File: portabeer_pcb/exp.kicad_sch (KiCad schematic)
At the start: 34 parts, among them J16 Conn_01x03, J18 Conn_02x05_Odd_Even, J4 Conn_01x08, M1 Air pump, Q6 SiS454DN, U12 PCA9536DP, U13 USBLC6-2SC6, U16 MCP47FEB12, U17 REF3012, U18 USBLC6-4SC6, U19 FDC1004DGST, U4 COS1416

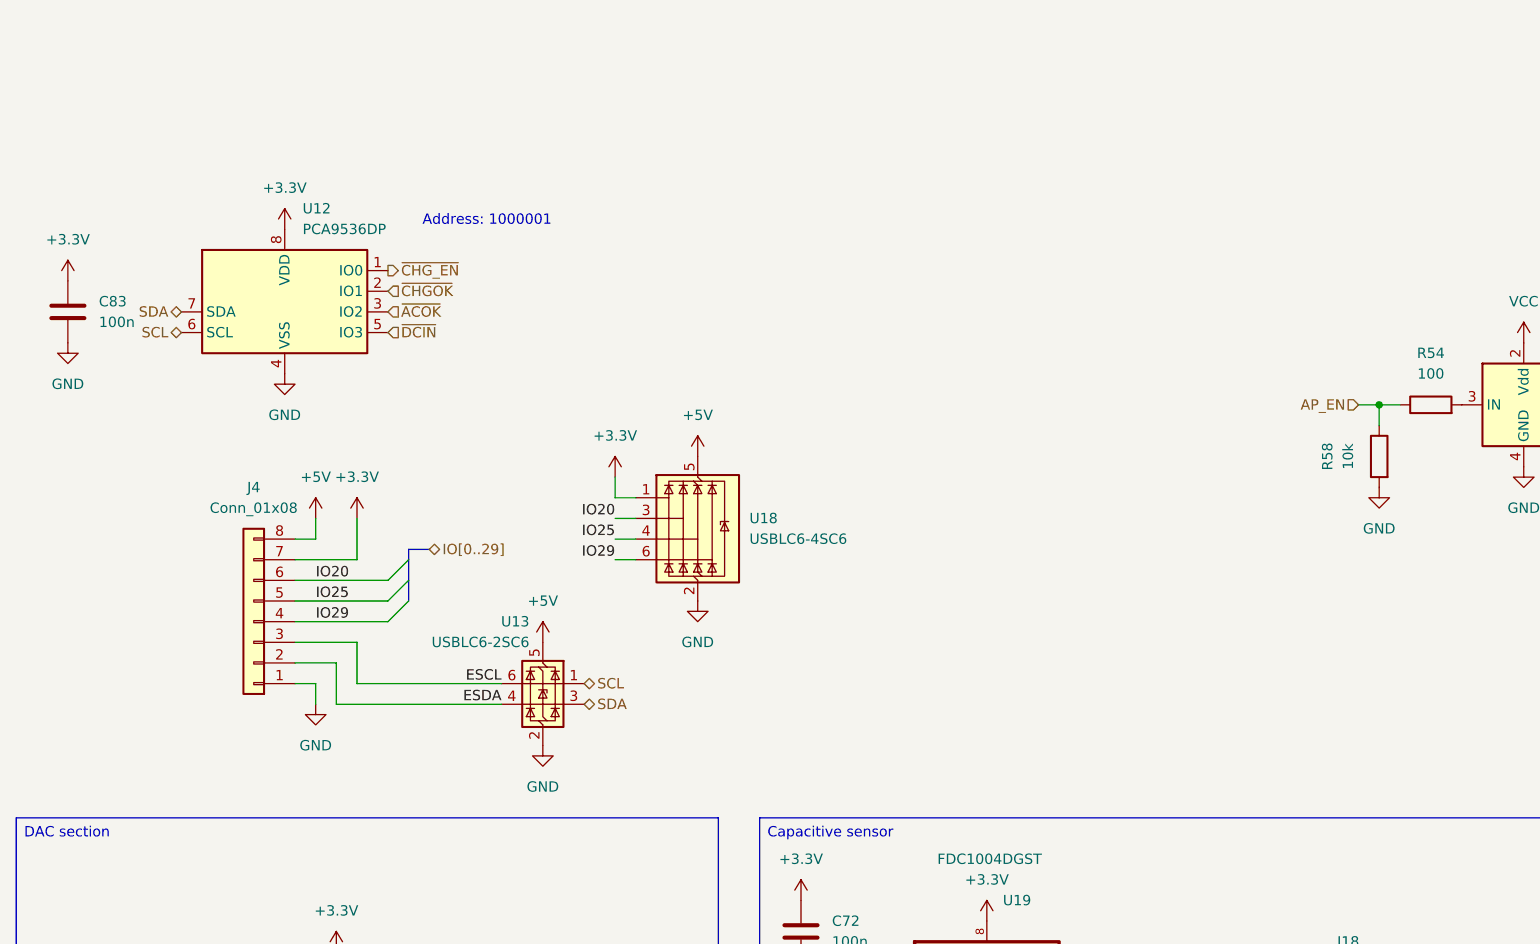
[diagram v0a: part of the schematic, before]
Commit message: layout
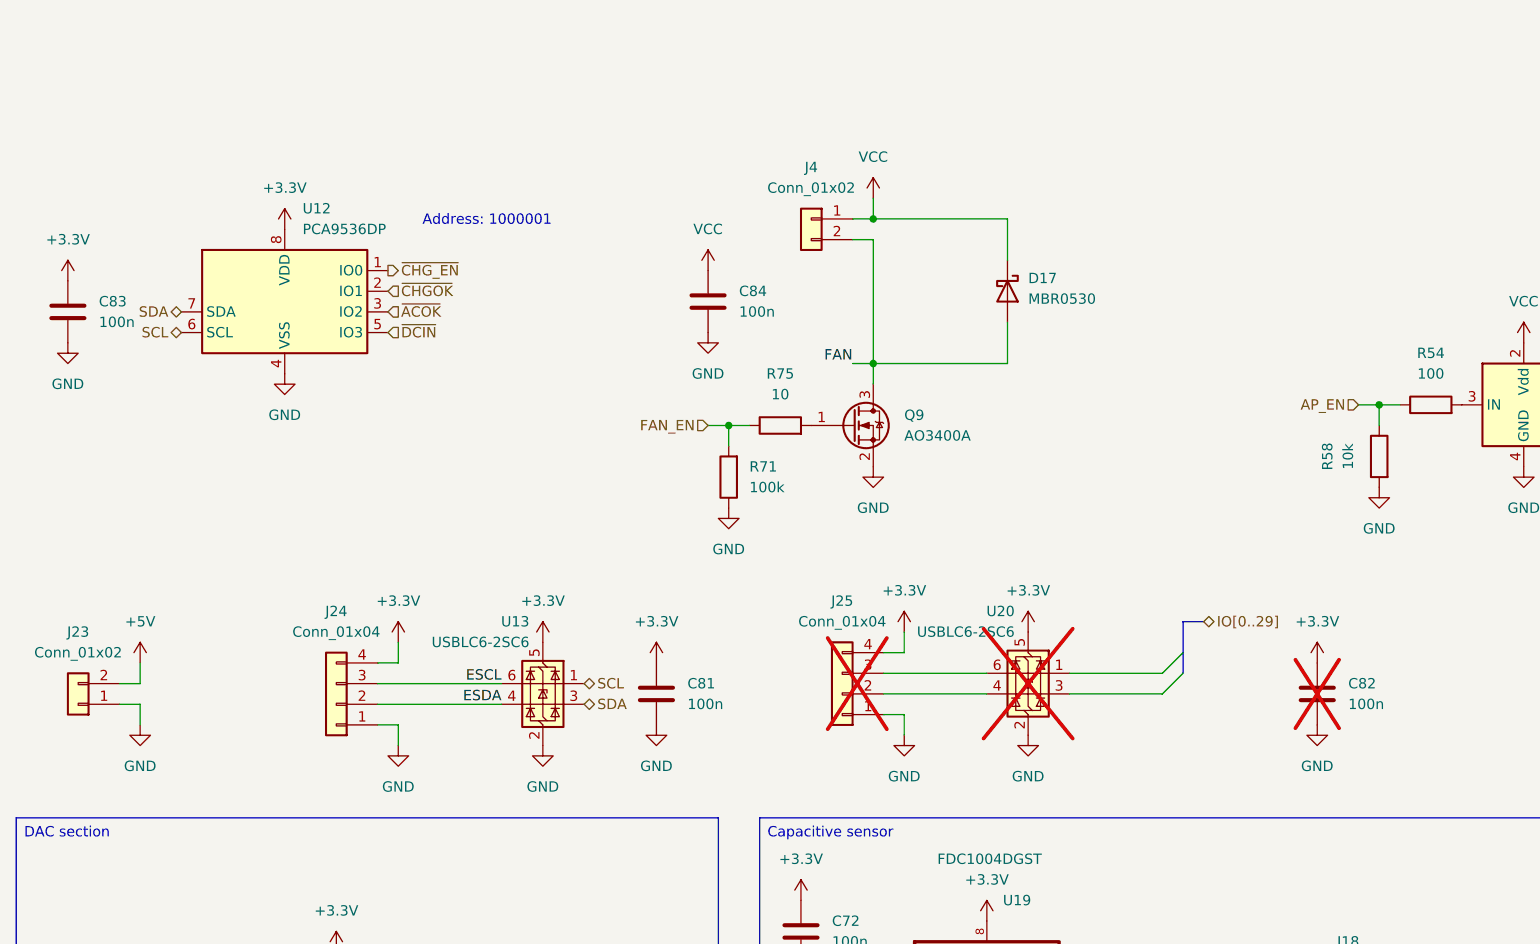
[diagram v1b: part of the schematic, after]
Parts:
- removed J4: Conn_01x08, Connector_PinHeader_2.54mm:PinHeader_1x08_P2.54mm_Vertical, symbol Connector_Generic:Conn_01x08
- removed U18: USBLC6-4SC6, Package_TO_SOT_SMD:SOT-23-6, symbol Power_Protection:USBLC6-4SC6
- added C81, C82, C84: 100n, Capacitor_SMD:C_0603_1608Metric, symbol Device:C
- added D17: MBR0530, Diode_SMD:D_SOD-123, symbol Diode:MBR0530
- added J23: Conn_01x02, Connector_PinHeader_2.54mm:PinHeader_1x02_P2.54mm_Vertical, symbol Connector_Generic:Conn_01x02
- added J24, J25: Conn_01x04, Connector_PinHeader_2.54mm:PinHeader_1x04_P2.54mm_Vertical, symbol Connector_Generic:Conn_01x04
- added J4: Conn_01x02, Connector_JST:JST_XH_S2B-XH-A_1x02_P2.50mm_Horizontal, symbol Connector_Generic:Conn_01x02
- added Q9: AO3400A, Package_TO_SOT_SMD:SOT-23, symbol Transistor_FET:AO3400A
- added R71: 100k, Resistor_SMD:R_0603_1608Metric, symbol Device:R
- added R75: 10, Resistor_SMD:R_0603_1608Metric, symbol Device:R
- added U20: USBLC6-2SC6, Package_TO_SOT_SMD:SOT-23-6, symbol Power_Protection:USBLC6-2SC6
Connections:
- net +3.3V: now also U13.5 (VBUS), C81.1, C82.1, J24.4 (Pin_4), J25.4 (Pin_4), U20.5 (VBUS)
- net +5V: now also J23.2 (Pin_2); no longer U13.5 (VBUS)
- net ESCL: now also J24.3 (Pin_3)
- net ESDA: now also J24.2 (Pin_2)
- net GND: now also C81.2, C82.2, C84.2, J23.1 (Pin_1), J24.1 (Pin_1), J25.1 (Pin_1), Q9.2 (S), R71.1, U20.2 (GND)
- net VCC: now also C84.1, D17.1 (K), J4.1 (Pin_1)
- new net: Q9.1 (G), R75.2
- new net: J25.2 (Pin_2), U20.4 (I/O2)
- new net: J25.3 (Pin_3), U20.6 (I/O1)
- new net FAN: D17.2 (A), J4.2 (Pin_2), Q9.3 (D)
- new net FAN_EN: R71.2, R75.1
